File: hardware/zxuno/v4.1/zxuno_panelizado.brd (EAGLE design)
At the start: 190 x 150 mm, 2 parts

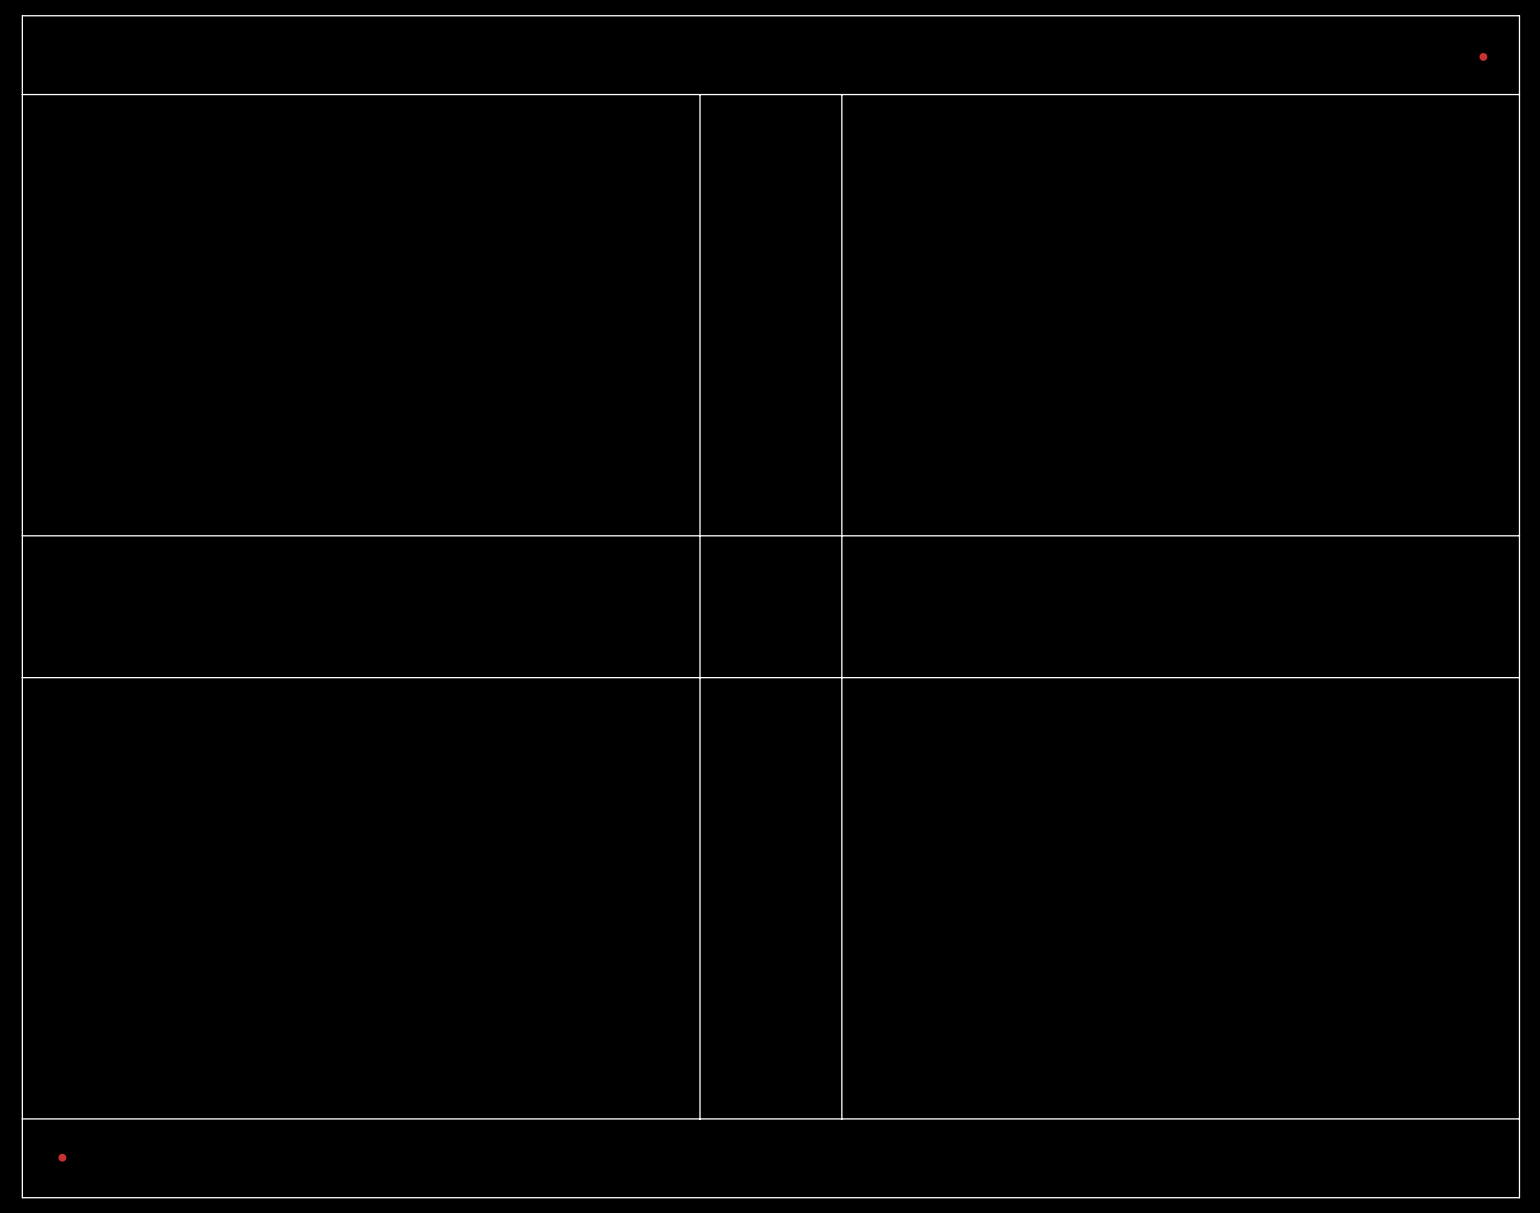
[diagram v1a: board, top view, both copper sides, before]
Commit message: Fin panelizado
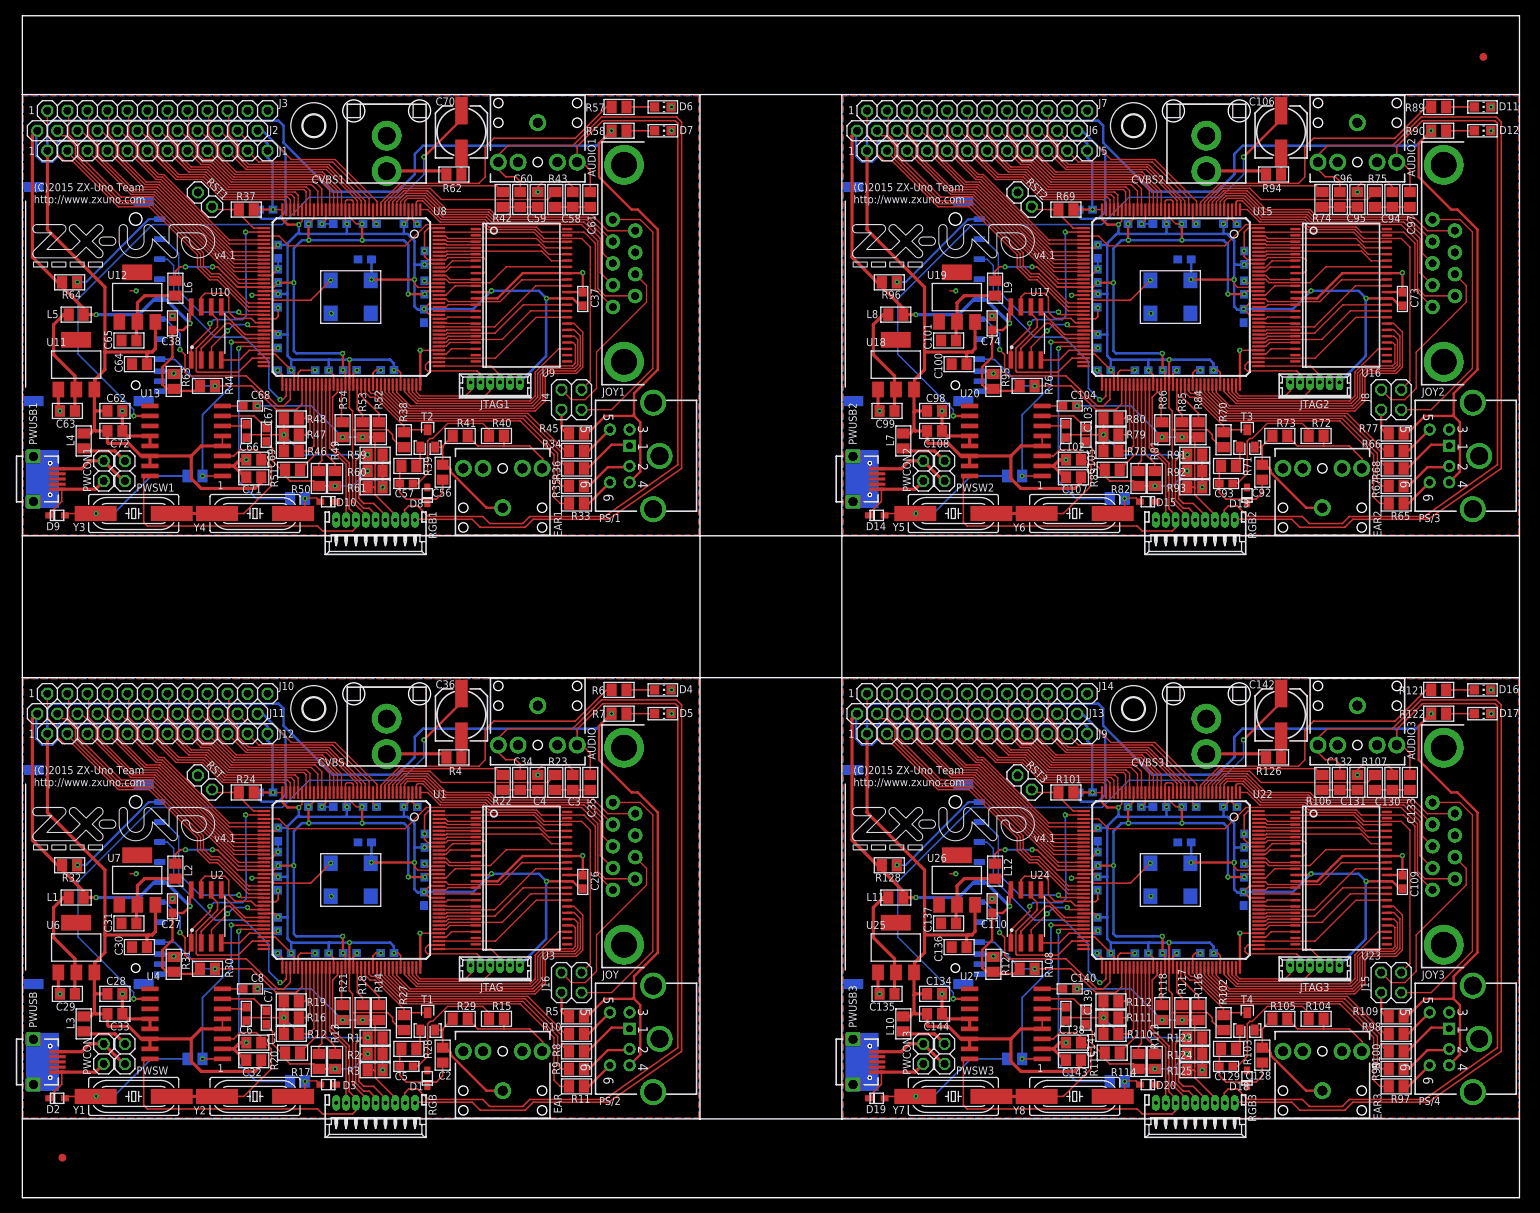
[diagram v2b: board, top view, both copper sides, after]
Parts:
- added AUDIO, AUDIO1, AUDIO2, AUDIO3: Audio, SparkFun-Connectors:AUDIO-JACK
- added C1, C105, C141, C69: 7.5pF, rcl:C0805
- added C10, C102, C103, C104, C109, C11, C110, C111, C112, C113, C114, C115, C116, C117, C118, C119, C12, C120, C121, C122, C123, C124, C125, C126, C127, C129, C13, C138, C139, C14, C140, C15, C16, C17, C18, C19, C20, C21, C22, C23, C24, C25, C26, C27, C37, C38, C39, C40, C41, C42, C43, C44, C45, C46, C47, C48, C49, C5, C50, C51, C52, C53, C54, C55, C57, C6, C66, C67, C68, C7, C73, C74, C75, C76, C77, C78, C79, C8, C80, C81, C82, C83, C84, C85, C86, C87, C88, C89, C9, C90, C91, C93: 100nF, rcl:C0603
- added C100, C101, C107, C108, C132, C133, C134, C135, C136, C137, C143, C144, C28, C29, C30, C31, C32, C33, C34, C35, C60, C61, C62, C63, C64, C65, C71, C72, C96, C97, C98, C99: 10uF, rcl:C0805
- added C106, C142, C36, C70: 220uF, rcl:153CLV-0605
- added C128, C130, C131, C2, C3, C4, C56, C58, C59, C92, C94, C95: 10nF, rcl:C0805
- added CVBS, CVBS1, CVBS2, CVBS3: RCA, uzebox:RCA
- added D1, D10, D13, D14, D15, D18, D19, D2, D20, D3, D8, D9: (no value), adafruit:SOD-323F
- added D11, D12, D16, D17, D4, D5, D6, D7: (no value), led:CHIP-LED0805
- added EAR, EAR1, EAR2, EAR3: EAR, SparkFun-Connectors:AUDIO-JACK
- added H1, H2, H3, H4: MOUNT-HOLE2.8, holes:2,8
- added J1, J10, J11, J12, J13, J14, J2, J3, J5, J6, J7, J9: (no value), pinhead:1X12
- added J15, J16, J4, J8: (no value), pinhead:2X02
- added JOY, JOY1, JOY2, JOY3: (no value), SparkFun-Connectors:DB9_MALE
- added JTAG, JTAG1, JTAG2, JTAG3: JTAG, con-molex:53047-06
- added L1, L10, L11, L12, L2, L3, L4, L5, L6, L7, L8, L9: (no value), rcl:M0805
- added PS/1, PS/2, PS/3, PS/4: PS/2 Keyb, ZX_UNO_0_14:DINC/MIN_TM/6_1PRIMARY
- added PWCON, PWCON1, PWCON2, PWCON3, PWSW, PWSW1, PWSW2, PWSW3, RST, RST1, RST2, RST3: (no value), pinhead:1X02
- added PWUSB, PWUSB1, PWUSB2, PWUSB3: MICROUSB, zxuno_rev_mcleod:MICRO_USB_1PRIMARY
- added R1, R123, R124, R125, R126, R2, R3, R4, R59, R60, R61, R62, R91, R92, R93, R94: 75, rcl:M0805
- added R10, R100, R104, R109, R11, R110, R113, R116, R12, R121, R122, R13, R14, R15, R33, R34, R35, R36, R40, R45, R46, R49, R5, R52, R57, R58, R6, R65, R66, R67, R68, R7, R72, R77, R78, R8, R81, R84, R89, R9, R90, R97, R98, R99: 510, rcl:M0805
- added R101, R106, R107, R112, R115, R118, R19, R20, R21, R22, R23, R24, R37, R42, R43, R48, R51, R54, R69, R74, R75, R80, R83, R86: 2K, rcl:M0805
- added R102, R103, R105, R108, R119, R120, R127, R128, R25, R26, R27, R28, R29, R30, R31, R32, R38, R39, R41, R44, R55, R56, R63, R64, R70, R71, R73, R76, R87, R88, R95, R96: 10K, rcl:M0805
- added R111, R114, R117, R16, R17, R18, R47, R50, R53, R79, R82, R85: 1K, rcl:M0805
- added RGB, RGB1, RGB2, RGB3: RGB, con-molex:53048-09
- added SDCARD, SDCARD1, SDCARD2, SDCARD3: (no value), zxuno_rev_mcleod:SDCMF-10915W010
- added T1, T2, T3, T4: BC846, transistor:SOT23
- added U1, U15, U22, U8: 6SLX9TQG144, xilinx_devices_V6:TQ144
- added U10, U17, U2, U24: FLASH-SPI-25XXSMD1, GadgetFactory:SO08-EIAJ
- added U11, U18, U25, U6: 3.3V, burr-brown:SOT223
- added U12, U19, U26, U7: 1.2V, burr-brown:SOT223
- added U13, U20, U27, U4: AD724, ad725:SO16W
- added U14, U21, U28, U5: 50MHz, ZX_UNO_0_15:SM/OSC_1PRIMARY
- added U16, U23, U3, U9: (no value), GadgetFactory:TSOP44-II
- added Y1, Y3, Y5, Y7: 3.58M, crystal:HC49UP
- added Y2, Y4, Y6, Y8: 4.43M, crystal:HC49UP
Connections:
- new net 1.2V: C10.2, C11.2, C12.2, C13.2, C9.2, L2.2, U1.P128, U1.P19, U1.P28, U1.P52, U1.P89
- new net 1.2V1: C39.2, C40.2, C41.2, C42.2, C43.2, L6.2, U8.P128, U8.P19, U8.P28, U8.P52, U8.P89
- new net 1.2V2: C75.2, C76.2, C77.2, C78.2, C79.2, L9.2, U15.P128, U15.P19, U15.P28, U15.P52, U15.P89
- new net 1.2V3: C111.2, C112.2, C113.2, C114.2, C115.2, L12.2, U22.P128, U22.P19, U22.P28, U22.P52, U22.P89
- new net 3.3V: C14.2, C15.2, C16.2, C17.2, C18.2, C19.2, C20.2, C21.2, C22.2, C23.2, C24.2, C25.2, C26.1, C27.2, J11.1, J12.12, JTAG.1, L1.2, R24.2, R27.2, R30.1, R31.2, R32.2, RGB.4, SDCARD.4, U1.P103, U1.P122, U1.P125, U1.P129, U1.P135, U1.P18, U1.P20, U1.P31, U1.P36, U1.P4, U1.P42, U1.P53, U1.P63, U1.P69, U1.P76, U1.P86, U1.P90, U2.8, U3.11, U3.33, U5.4
- new net 3.3V1: C37.1, C38.2, C44.2, C45.2, C46.2, C47.2, C48.2, C49.2, C50.2, C51.2, C52.2, C53.2, C54.2, C55.2, J1.12, J2.1, JTAG1.1, L5.2, R37.2, R38.2, R44.1, R63.2, R64.2, RGB1.4, SDCARD1.4, U10.8, U14.4, U8.P103, U8.P122, U8.P125, U8.P129, U8.P135, U8.P18, U8.P20, U8.P31, U8.P36, U8.P4, U8.P42, U8.P53, U8.P63, U8.P69, U8.P76, U8.P86, U8.P90, U9.11, U9.33
- new net 3.3V2: C73.1, C74.2, C80.2, C81.2, C82.2, C83.2, C84.2, C85.2, C86.2, C87.2, C88.2, C89.2, C90.2, C91.2, J5.12, J6.1, JTAG2.1, L8.2, R69.2, R70.2, R76.1, R95.2, R96.2, RGB2.4, SDCARD2.4, U15.P103, U15.P122, U15.P125, U15.P129, U15.P135, U15.P18, U15.P20, U15.P31, U15.P36, U15.P4, U15.P42, U15.P53, U15.P63, U15.P69, U15.P76, U15.P86, U15.P90, U16.11, U16.33, U17.8, U21.4
- new net 3.3V3: C109.1, C110.2, C116.2, C117.2, C118.2, C119.2, C120.2, C121.2, C122.2, C123.2, C124.2, C125.2, C126.2, C127.2, J13.1, J9.12, JTAG3.1, L11.2, R101.2, R102.2, R108.1, R127.2, R128.2, RGB3.4, SDCARD3.4, U22.P103, U22.P122, U22.P125, U22.P129, U22.P135, U22.P18, U22.P20, U22.P31, U22.P36, U22.P4, U22.P42, U22.P53, U22.P63, U22.P69, U22.P76, U22.P86, U22.P90, U23.11, U23.33, U24.8, U28.4
- new net 5V: C28.1, C30.1, C32.2, C33.2, J12.1, L3.2, PS/2.4, R5.1, R7.2, U4.14, U4.15, U4.4, U4.5, U6.3, U7.3
- new net 5V1: C62.1, C64.1, C71.2, C72.2, J1.1, L4.2, PS/1.4, R45.1, R58.2, U11.3, U12.3, U13.14, U13.15, U13.4, U13.5
- new net 5V2: C100.1, C107.2, C108.2, C98.1, J5.1, L7.2, PS/3.4, R77.1, R90.2, U18.3, U19.3, U20.14, U20.15, U20.4, U20.5
- new net 5V3: C134.1, C136.1, C143.2, C144.2, J9.1, L10.2, PS/4.4, R109.1, R122.2, U25.3, U26.3, U27.14, U27.15, U27.4, U27.5
- new net AUDIO_LEFT: R22.2, U1.P10
- new net AUDIO_LEFT1: R42.2, U8.P10
- new net AUDIO_LEFT2: R74.2, U15.P10
- new net AUDIO_LEFT3: R106.2, U22.P10
- new net AUDIO_RIGHT: R23.2, U1.P9
- new net AUDIO_RIGHT1: R43.2, U8.P9
- new net AUDIO_RIGHT2: R75.2, U15.P9
- new net AUDIO_RIGHT3: R107.2, U22.P9
- new net B: C8.2, R14.1, R18.1, R21.1, R3.1, RGB.7
- new net B0: R21.2, U1.P88
- new net B1: R18.2, U1.P92
- new net B10: C104.2, R84.1, R85.1, R86.1, R93.1, RGB2.7
- new net B11: R118.2, U22.P88
- new net B12: R117.2, U22.P92
- new net B13: R116.2, U22.P93
- new net B14: C140.2, R116.1, R117.1, R118.1, R125.1, RGB3.7
- new net B2: R14.2, U1.P93
- new net B3: R54.2, U8.P88
- new net B4: R53.2, U8.P92
- new net B5: R52.2, U8.P93
- new net B6: C68.2, R52.1, R53.1, R54.1, R61.1, RGB1.7
- new net B7: R86.2, U15.P88
- new net B8: R85.2, U15.P92
- new net B9: R84.2, U15.P93
- new net CLK: U1.P55, U5.3
- new net CLK1: U14.3, U8.P55
- new net CLK2: U15.P55, U21.3
- new net CLK3: U22.P55, U28.3
- new net CSYNC: RGB.3, U1.P87, U4.16
- new net CSYNC1: RGB1.3, U13.16, U8.P87
- new net CSYNC2: RGB2.3, U15.P87, U20.16
- new net CSYNC3: RGB3.3, U22.P87, U27.16
- new net EAR: R27.1, T1.3, U1.P94
- new net EAR1: R38.1, T2.3, U8.P94
- new net EAR2: R70.1, T3.3, U15.P94
- new net EAR3: R102.1, T4.3, U22.P94
- new net EXT1: J1.2, U8.P57
- new net EXT10: J12.3, U1.P50
- new net EXT100: J9.5, U22.P43
- new net EXT101: J13.5, U22.P41
- new net EXT102: J14.5, U22.P40
- new net EXT103: J9.6, U22.P35
- new net EXT104: J13.6, U22.P34
- new net EXT105: J14.6, U22.P33
- new net EXT106: J9.7, U22.P32
- new net EXT107: J13.7, U22.P30
- new net EXT108: J14.7, U22.P29
- new net EXT109: J9.8, U22.P27
- new net EXT11: J11.3, U1.P48
- new net EXT110: J13.8, U22.P26
- new net EXT111: J14.8, U22.P24
- new net EXT112: J9.9, U22.P23
- new net EXT113: J13.9, U22.P22
- new net EXT114: J14.9, U22.P21
- new net EXT115: J9.10, U22.P17
- new net EXT116: J13.10, U22.P16
- new net EXT117: J14.10, U22.P15
- new net EXT118: J9.11, U22.P14
- new net EXT119: J13.11, U22.P12
- new net EXT12: J10.3, U1.P47
- new net EXT120: J14.1, U22.P58
- new net EXT13: J12.4, U1.P46
- new net EXT14: J11.4, U1.P45
- new net EXT15: J10.4, U1.P44
- new net EXT16: J12.5, U1.P43
- new net EXT17: J11.5, U1.P41
- new net EXT18: J10.5, U1.P40
- new net EXT19: J12.6, U1.P35
- new net EXT2: J2.2, U8.P56
- new net EXT20: J11.6, U1.P34
- new net EXT21: J10.6, U1.P33
- new net EXT22: J12.7, U1.P32
- new net EXT23: J11.7, U1.P30
- new net EXT24: J10.7, U1.P29
- new net EXT25: J12.8, U1.P27
- new net EXT26: J11.8, U1.P26
- new net EXT27: J10.8, U1.P24
- new net EXT28: J12.9, U1.P23
- new net EXT29: J11.9, U1.P22
- new net EXT3: J3.2, U8.P51
- new net EXT30: J10.9, U1.P21
- new net EXT31: J12.10, U1.P17
- new net EXT32: J11.10, U1.P16
- new net EXT33: J10.10, U1.P15
- new net EXT34: J12.11, U1.P14
- new net EXT35: J11.11, U1.P12
- new net EXT36: J3.3, U8.P47
- new net EXT37: J1.4, U8.P46
- new net EXT38: J2.4, U8.P45
- new net EXT39: J3.4, U8.P44
- new net EXT4: J1.3, U8.P50
- new net EXT40: J1.5, U8.P43
- new net EXT41: J2.5, U8.P41
- new net EXT42: J3.5, U8.P40
- new net EXT43: J1.6, U8.P35
- new net EXT44: J2.6, U8.P34
- new net EXT45: J3.6, U8.P33
- new net EXT46: J1.7, U8.P32
- new net EXT47: J2.7, U8.P30
- new net EXT48: J3.7, U8.P29
- new net EXT49: J1.8, U8.P27
- new net EXT5: J2.3, U8.P48
- new net EXT50: J2.8, U8.P26
- new net EXT51: J3.8, U8.P24
- new net EXT52: J1.9, U8.P23
- new net EXT53: J2.9, U8.P22
- new net EXT54: J3.9, U8.P21
- new net EXT55: J1.10, U8.P17
- new net EXT56: J2.10, U8.P16
- new net EXT57: J3.10, U8.P15
- new net EXT58: J1.11, U8.P14
- new net EXT59: J2.11, U8.P12
- new net EXT6: J10.1, U1.P58
- new net EXT60: J3.1, U8.P58
- new net EXT61: J5.2, U15.P57
- new net EXT62: J6.2, U15.P56
- new net EXT63: J7.2, U15.P51
- new net EXT64: J5.3, U15.P50
- new net EXT65: J6.3, U15.P48
- new net EXT66: J7.3, U15.P47
- new net EXT67: J5.4, U15.P46
- new net EXT68: J6.4, U15.P45
- new net EXT69: J7.4, U15.P44
- new net EXT7: J12.2, U1.P57
- new net EXT70: J5.5, U15.P43
- new net EXT71: J6.5, U15.P41
- new net EXT72: J7.5, U15.P40
- new net EXT73: J5.6, U15.P35
- new net EXT74: J6.6, U15.P34
- new net EXT75: J7.6, U15.P33
- new net EXT76: J5.7, U15.P32
- new net EXT77: J6.7, U15.P30
- new net EXT78: J7.7, U15.P29
- new net EXT79: J5.8, U15.P27
- new net EXT8: J11.2, U1.P56
- new net EXT80: J6.8, U15.P26
- new net EXT81: J7.8, U15.P24
- new net EXT82: J5.9, U15.P23
- new net EXT83: J6.9, U15.P22
- new net EXT84: J7.9, U15.P21
- new net EXT85: J5.10, U15.P17
- new net EXT86: J6.10, U15.P16
- new net EXT87: J7.10, U15.P15
- new net EXT88: J5.11, U15.P14
- new net EXT89: J6.11, U15.P12
- new net EXT9: J10.2, U1.P51
- new net EXT90: J7.1, U15.P58
- new net EXT91: J9.2, U22.P57
- new net EXT92: J13.2, U22.P56
- new net EXT93: J14.2, U22.P51
- new net EXT94: J9.3, U22.P50
- new net EXT95: J13.3, U22.P48
- new net EXT96: J14.3, U22.P47
- new net EXT97: J9.4, U22.P46
- new net EXT98: J13.4, U22.P45
- new net EXT99: J14.4, U22.P44
- new net FLASH_CS: U1.P38, U2.1
- new net FLASH_CS1: U10.1, U8.P38
- new net FLASH_CS2: U15.P38, U17.1
- new net FLASH_CS3: U22.P38, U24.1
- new net FLASH_HOLD: U1.P61, U2.7
- new net FLASH_HOLD1: U10.7, U8.P61
- new net FLASH_HOLD2: U15.P61, U17.7
- new net FLASH_HOLD3: U22.P61, U24.7
- new net FLASH_MISO: U1.P65, U2.2
- new net FLASH_MISO1: U10.2, U8.P65
- new net FLASH_MISO2: U15.P65, U17.2
- new net FLASH_MISO3: U22.P65, U24.2
- new net FLASH_MOSI: U1.P64, U2.5
- new net FLASH_MOSI1: U10.5, U8.P64
- new net FLASH_MOSI2: U15.P64, U17.5
- new net FLASH_MOSI3: U22.P64, U24.5
- new net FLASH_SCK: U1.P70, U2.6
- new net FLASH_SCK1: U10.6, U8.P70
- new net FLASH_SCK2: U15.P70, U17.6
- new net FLASH_SCK3: U22.P70, U24.6
- new net FLASH_WP: U1.P62, U2.3
- new net FLASH_WP1: U10.3, U8.P62
- new net FLASH_WP2: U15.P62, U17.3
- new net FLASH_WP3: U22.P62, U24.3
- new net G: C7.2, R13.1, R17.1, R2.1, R20.1, RGB.6
- new net G0: R20.2, U1.P82
- new net G1: R17.2, U1.P83
- new net G10: C103.2, R81.1, R82.1, R83.1, R92.1, RGB2.6
- new net G11: R115.2, U22.P82
- new net G12: R114.2, U22.P83
- new net G13: R113.2, U22.P84
- new net G14: C139.2, R113.1, R114.1, R115.1, R124.1, RGB3.6
- new net G2: R13.2, U1.P84
- new net G3: R51.2, U8.P82
- new net G4: R50.2, U8.P83
- new net G5: R49.2, U8.P84
- new net G6: C67.2, R49.1, R50.1, R51.1, R60.1, RGB1.6
- new net G7: R83.2, U15.P82
- new net G8: R82.2, U15.P83
- new net G9: R81.2, U15.P84
- new net GND: AUDIO.SLEEVE, C1.2, C10.1, C11.1, C12.1, C13.1, C14.1, C15.1, C16.1, C17.1, C18.1, C19.1, C2.2, C20.1, C21.1, C22.1, C23.1, C24.1, C25.1, C26.2, C27.1, C28.2, C29.2, C3.2, C30.2, C31.2, C32.1, C33.1, C4.2, C9.1, CVBS.GND, D1.A, D2.C, D3.C, D4.C, D5.C, EAR.SLEEVE, J10.12, J11.12, JOY.8, JTAG.2, PS/2.3, PWCON.1, PWUSB.5, R1.2, R2.2, R29.2, R3.2, RGB.1, RST.1, SDCARD.3, SDCARD.6, SDCARD.M1, SDCARD.M2, SDCARD.M3, SDCARD.M4, T1.2, U1.P108, U1.P113, U1.P13, U1.P130, U1.P136, U1.P144, U1.P25, U1.P3, U1.P49, U1.P54, U1.P60, U1.P68, U1.P73, U1.P77, U1.P91, U1.P96, U2.4, U3.12, U3.34, U3.37, U3.8, U4.12, U4.13, U4.2, U5.2, U6.1, U7.1
- new net GND1: AUDIO1.SLEEVE, C37.2, C38.1, C39.1, C40.1, C41.1, C42.1, C43.1, C44.1, C45.1, C46.1, C47.1, C48.1, C49.1, C50.1, C51.1, C52.1, C53.1, C54.1, C55.1, C56.2, C58.2, C59.2, C62.2, C63.2, C64.2, C65.2, C69.2, C71.1, C72.1, CVBS1.GND, D10.C, D6.C, D7.C, D8.A, D9.C, EAR1.SLEEVE, J2.12, J3.12, JOY1.8, JTAG1.2, PS/1.3, PWCON1.1, PWUSB1.5, R41.2, R59.2, R60.2, R61.2, RGB1.1, RST1.1, SDCARD1.3, SDCARD1.6, SDCARD1.M1, SDCARD1.M2, SDCARD1.M3, SDCARD1.M4, T2.2, U10.4, U11.1, U12.1, U13.12, U13.13, U13.2, U14.2, U8.P108, U8.P113, U8.P13, U8.P130, U8.P136, U8.P144, U8.P25, U8.P3, U8.P49, U8.P54, U8.P60, U8.P68, U8.P73, U8.P77, U8.P91, U8.P96, U9.12, U9.34, U9.37, U9.8
- new net GND2: AUDIO2.SLEEVE, C100.2, C101.2, C105.2, C107.1, C108.1, C73.2, C74.1, C75.1, C76.1, C77.1, C78.1, C79.1, C80.1, C81.1, C82.1, C83.1, C84.1, C85.1, C86.1, C87.1, C88.1, C89.1, C90.1, C91.1, C92.2, C94.2, C95.2, C98.2, C99.2, CVBS2.GND, D11.C, D12.C, D13.A, D14.C, D15.C, EAR2.SLEEVE, J6.12, J7.12, JOY2.8, JTAG2.2, PS/3.3, PWCON2.1, PWUSB2.5, R73.2, R91.2, R92.2, R93.2, RGB2.1, RST2.1, SDCARD2.3, SDCARD2.6, SDCARD2.M1, SDCARD2.M2, SDCARD2.M3, SDCARD2.M4, T3.2, U15.P108, U15.P113, U15.P13, U15.P130, U15.P136, U15.P144, U15.P25, U15.P3, U15.P49, U15.P54, U15.P60, U15.P68, U15.P73, U15.P77, U15.P91, U15.P96, U16.12, U16.34, U16.37, U16.8, U17.4, U18.1, U19.1, U20.12, U20.13, U20.2, U21.2
- new net GND3: AUDIO3.SLEEVE, C109.2, C110.1, C111.1, C112.1, C113.1, C114.1, C115.1, C116.1, C117.1, C118.1, C119.1, C120.1, C121.1, C122.1, C123.1, C124.1, C125.1, C126.1, C127.1, C128.2, C130.2, C131.2, C134.2, C135.2, C136.2, C137.2, C141.2, C143.1, C144.1, CVBS3.GND, D16.C, D17.C, D18.A, D19.C, D20.C, EAR3.SLEEVE, J13.12, J14.12, JOY3.8, JTAG3.2, PS/4.3, PWCON3.1, PWUSB3.5, R105.2, R123.2, R124.2, R125.2, RGB3.1, RST3.1, SDCARD3.3, SDCARD3.6, SDCARD3.M1, SDCARD3.M2, SDCARD3.M3, SDCARD3.M4, T4.2, U22.P108, U22.P113, U22.P13, U22.P130, U22.P136, U22.P144, U22.P25, U22.P3, U22.P49, U22.P54, U22.P60, U22.P68, U22.P73, U22.P77, U22.P91, U22.P96, U23.12, U23.34, U23.37, U23.8, U24.4, U25.1, U26.1, U27.12, U27.13, U27.2, U28.2
- new net JOY_DOWN: JOY.2, U1.P5
- new net JOY_DOWN1: JOY1.2, U8.P5
- new net JOY_DOWN2: JOY2.2, U15.P5
- new net JOY_DOWN3: JOY3.2, U22.P5
- new net JOY_FIRE1: JOY.6, U1.P2
- new net JOY_FIRE10: JOY3.6, U22.P2
- new net JOY_FIRE11: JOY3.9, U22.P8
- new net JOY_FIRE12: J15.1, U22.P39
- new net JOY_FIRE2: JOY.9, U1.P8
- new net JOY_FIRE3: J16.1, U1.P39
- new net JOY_FIRE4: JOY1.6, U8.P2
- new net JOY_FIRE5: JOY1.9, U8.P8
- new net JOY_FIRE6: J4.1, U8.P39
- new net JOY_FIRE7: JOY2.6, U15.P2
- new net JOY_FIRE8: JOY2.9, U15.P8
- new net JOY_FIRE9: J8.1, U15.P39
- new net JOY_LEFT: JOY.3, U1.P6
- new net JOY_LEFT1: JOY1.3, U8.P6
- new net JOY_LEFT2: JOY2.3, U15.P6
- new net JOY_LEFT3: JOY3.3, U22.P6
- new net JOY_RIGHT: JOY.4, U1.P7
- new net JOY_RIGHT1: JOY1.4, U8.P7
- new net JOY_RIGHT2: JOY2.4, U15.P7
- new net JOY_RIGHT3: JOY3.4, U22.P7
- new net JOY_UP: JOY.1, U1.P1
- new net JOY_UP1: JOY1.1, U8.P1
- new net JOY_UP2: JOY2.1, U15.P1
- new net JOY_UP3: JOY3.1, U22.P1
- new net L-OUT: AUDIO.TIP, C34.2, RGB.9
- new net L-OUT1: AUDIO1.TIP, C60.2, RGB1.9
- new net L-OUT2: AUDIO2.TIP, C96.2, RGB2.9
- new net L-OUT3: AUDIO3.TIP, C132.2, RGB3.9
- new net LED: R6.2, U1.P11
- new net LED1: R57.2, U8.P11
- new net LED2: R89.2, U15.P11
- new net LED3: R121.2, U22.P11
- new net N$1: PS/2.6, R11.1
- new net N$10: C3.1, C35.1, R23.1
- new net N$100: C135.1, L11.1, U25.2
- new net N$101: C137.1, L12.1, U26.2
- new net N$102: C139.1, U27.7
- new net N$103: C138.1, U27.6
- new net N$104: C141.1, U27.3, Y7.2, Y8.2
- new net N$105: D20.A, R120.1, Y8.1
- new net N$106: D19.A, R119.2, Y7.1
- new net N$107: C142.+, U27.10
- new net N$108: C140.1, U27.8
- new net N$109: C142.-, R126.1
- new net N$11: C34.1, C4.1, R22.1
- new net N$110: CVBS3.SIG, R126.2
- new net N$111: D16.A, R121.1
- new net N$112: D17.A, R122.1
- new net N$113: R101.1, RST3.2, U22.P37
- new net N$114: R127.1, SDCARD3.8
- new net N$115: R128.1, SDCARD3.9
- new net N$116: J15.4, R109.2
- new net N$12: PWCON.2, PWSW.2, PWUSB.1
- new net N$13: L3.1, PWSW.1
- new net N$14: C29.1, L1.1, U6.2
- new net N$15: J16.4, R5.2
- new net N$16: PS/1.6, R33.1
- new net N$17: C31.1, L2.1, U7.2
- new net N$18: R31.1, SDCARD.8
- new net N$19: C8.1, U4.8
- new net N$2: PS/2.5, R10.1
- new net N$20: R32.1, SDCARD.9
- new net N$21: C7.1, U4.7
- new net N$22: C6.1, U4.6
- new net N$23: C1.1, U4.3, Y1.2, Y2.2
- new net N$24: D3.A, R26.1, Y2.1
- new net N$25: D2.A, R25.2, Y1.1
- new net N$26: C36.+, U4.10
- new net N$27: C36.-, R4.1
- new net N$28: CVBS.SIG, R4.2
- new net N$29: PS/1.5, R34.1
- new net N$3: PS/2.2, R9.1
- new net N$30: PS/1.2, R35.1
- new net N$31: D4.A, R6.1
- new net N$32: D5.A, R7.1
- new net N$33: PS/1.1, R36.1
- new net N$34: R39.2, T2.1
- new net N$35: C56.1, C57.1, D8.C, R39.1
- new net N$36: C57.2, R40.2
- new net N$37: EAR1.TIP, R40.1, R41.1
- new net N$38: C58.1, C61.1, R43.1
- new net N$39: C59.1, C60.1, R42.1
- new net N$4: PS/2.1, R8.1
- new net N$40: PWCON1.2, PWSW1.2, PWUSB1.1
- new net N$41: L4.1, PWSW1.1
- new net N$42: C63.1, L5.1, U11.2
- new net N$43: C65.1, L6.1, U12.2
- new net N$44: C67.1, U13.7
- new net N$45: C66.1, U13.6
- new net N$46: C69.1, U13.3, Y3.2, Y4.2
- new net N$47: D10.A, R56.1, Y4.1
- new net N$48: D9.A, R55.2, Y3.1
- new net N$49: C70.+, U13.10
- new net N$5: R24.1, RST.2, U1.P37
- new net N$50: C68.1, U13.8
- new net N$51: C70.-, R62.1
- new net N$52: CVBS1.SIG, R62.2
- new net N$53: D6.A, R57.1
- new net N$54: D7.A, R58.1
- new net N$55: R37.1, RST1.2, U8.P37
- new net N$56: R63.1, SDCARD1.8
- new net N$57: R64.1, SDCARD1.9
- new net N$58: J4.4, R45.2
- new net N$59: PS/3.6, R65.1
- new net N$6: R28.2, T1.1
- new net N$60: PS/3.5, R66.1
- new net N$61: PS/3.2, R67.1
- new net N$62: PS/3.1, R68.1
- new net N$63: R71.2, T3.1
- new net N$64: C92.1, C93.1, D13.C, R71.1
- new net N$65: C93.2, R72.2
- new net N$66: EAR2.TIP, R72.1, R73.1
- new net N$67: C94.1, C97.1, R75.1
- new net N$68: C95.1, C96.1, R74.1
- new net N$69: PWCON2.2, PWSW2.2, PWUSB2.1
- new net N$7: C2.1, C5.1, D1.C, R28.1
- new net N$70: L7.1, PWSW2.1
- new net N$71: C99.1, L8.1, U18.2
- new net N$72: C101.1, L9.1, U19.2
- new net N$73: C103.1, U20.7
- new net N$74: C102.1, U20.6
- new net N$75: C105.1, U20.3, Y5.2, Y6.2
- new net N$76: D15.A, R88.1, Y6.1
- new net N$77: D14.A, R87.2, Y5.1
- new net N$78: C106.+, U20.10
- new net N$79: C104.1, U20.8
- new net N$8: C5.2, R15.2
- new net N$80: C106.-, R94.1
- new net N$81: CVBS2.SIG, R94.2
- new net N$82: D11.A, R89.1
- new net N$83: D12.A, R90.1
- new net N$84: R69.1, RST2.2, U15.P37
- new net N$85: R95.1, SDCARD2.8
- new net N$86: R96.1, SDCARD2.9
- new net N$87: J8.4, R77.2
- new net N$88: PS/4.6, R97.1
- new net N$89: PS/4.5, R98.1
- new net N$9: EAR.TIP, R15.1, R29.1
- new net N$90: PS/4.2, R99.1
- new net N$91: PS/4.1, R100.1
- new net N$92: R103.2, T4.1
- new net N$93: C128.1, C129.1, D18.C, R103.1
- new net N$94: C129.2, R104.2
- new net N$95: EAR3.TIP, R104.1, R105.1
- new net N$96: C130.1, C133.1, R107.1
- new net N$97: C131.1, C132.1, R106.1
- new net N$98: PWCON3.2, PWSW3.2, PWUSB3.1
- new net N$99: L10.1, PWSW3.1
- new net PIN1: J4.3, JOY1.7
- new net PIN2: J4.2, JOY1.5
- new net PIN3: J8.3, JOY2.7
- new net PIN4: J8.2, JOY2.5
- new net PIN5: J16.2, JOY.5
- new net PIN6: J15.3, JOY3.7
- new net PIN7: J16.3, JOY.7
- new net PIN8: J15.2, JOY3.5
- new net PS2_CLK: R10.2, U1.P99
- new net PS2_CLK1: R34.2, U8.P99
- new net PS2_CLK2: R66.2, U15.P99
- new net PS2_CLK3: R98.2, U22.P99
- new net PS2_DATA: R8.2, U1.P98
- new net PS2_DATA1: R36.2, U8.P98
- new net PS2_DATA2: R68.2, U15.P98
- new net PS2_DATA3: R100.2, U22.P98
- new net PS2_PIN1: R33.2, U8.P95
- new net PS2_PIN2: R9.2, U1.P97
- new net PS2_PIN3: R35.2, U8.P97
- new net PS2_PIN4: R65.2, U15.P95
- new net PS2_PIN5: R67.2, U15.P97
- new net PS2_PIN6: R11.2, U1.P95
- new net PS2_PIN7: R97.2, U22.P95
- new net PS2_PIN8: R99.2, U22.P97
- new net R: C6.2, R1.1, R12.1, R16.1, R19.1, RGB.5
- new net R-OUT: AUDIO.RING, C35.2, RGB.8
- new net R-OUT1: AUDIO1.RING, C61.2, RGB1.8
- new net R-OUT2: AUDIO2.RING, C97.2, RGB2.8
- new net R-OUT3: AUDIO3.RING, C133.2, RGB3.8
- new net R0: R19.2, U1.P79
- new net R1: R16.2, U1.P80
- new net R10: C102.2, R78.1, R79.1, R80.1, R91.1, RGB2.5
- new net R11: R112.2, U22.P79
- new net R12: R111.2, U22.P80
- new net R13: R110.2, U22.P81
- new net R14: C138.2, R110.1, R111.1, R112.1, R123.1, RGB3.5
- new net R2: R12.2, U1.P81
- new net R3: R48.2, U8.P79
- new net R4: R47.2, U8.P80
- new net R5: R46.2, U8.P81
- new net R6: C66.2, R46.1, R47.1, R48.1, R59.1, RGB1.5
- new net R7: R80.2, U15.P79
- new net R8: R79.2, U15.P80
- new net R9: R78.2, U15.P81
- new net SD_CS: SDCARD.1, U1.P59
- new net SD_CS1: SDCARD1.1, U8.P59
- new net SD_CS2: SDCARD2.1, U15.P59
- new net SD_CS3: SDCARD3.1, U22.P59
- new net SD_MISO: R30.2, SDCARD.7, U1.P78
- new net SD_MISO1: R44.2, SDCARD1.7, U8.P78
- new net SD_MISO2: R76.2, SDCARD2.7, U15.P78
- new net SD_MISO3: R108.2, SDCARD3.7, U22.P78
- new net SD_MOSI: SDCARD.2, U1.P74
- new net SD_MOSI1: SDCARD1.2, U8.P74
- new net SD_MOSI2: SDCARD2.2, U15.P74
- new net SD_MOSI3: SDCARD3.2, U22.P74
- new net SD_SCK: SDCARD.5, U1.P75
- new net SD_SCK1: SDCARD1.5, U8.P75
- new net SD_SCK2: SDCARD2.5, U15.P75
- new net SD_SCK3: SDCARD3.5, U22.P75
- new net STDN: R25.1, U1.P66, U4.1
- new net STDN1: R55.1, U13.1, U8.P66
- new net STDN2: R87.1, U15.P66, U20.1
- new net STDN3: R119.1, U22.P66, U27.1
- new net STDNB: R26.2, U1.P67
- new net STDNB1: R56.2, U8.P67
- new net STDNB2: R88.2, U15.P67
- new net STDNB3: R120.2, U22.P67
- new net TCK: JTAG.3, U1.P109
- new net TCK1: JTAG1.3, U8.P109
- new net TCK2: JTAG2.3, U15.P109
- new net TCK3: JTAG3.3, U22.P109
- new net TDI: JTAG.5, U1.P110
- new net TDI1: JTAG1.5, U8.P110
- new net TDI2: JTAG2.5, U15.P110
- new net TDI3: JTAG3.5, U22.P110
- new net TDO: JTAG.4, U1.P106
- new net TDO1: JTAG1.4, U8.P106
- new net TDO2: JTAG2.4, U15.P106
- new net TDO3: JTAG3.4, U22.P106
- new net TMS: JTAG.6, U1.P107
- new net TMS1: JTAG1.6, U8.P107
- new net TMS2: JTAG2.6, U15.P107
- new net TMS3: JTAG3.6, U22.P107
- new net VSYNC: RGB.2, U1.P85
- new net VSYNC1: RGB1.2, U8.P85
- new net VSYNC2: RGB2.2, U15.P85
- new net VSYNC3: RGB3.2, U22.P85
- new net WR: U1.P121, U3.15
- new net WR1: U8.P121, U9.15
- new net WR2: U15.P121, U16.15
- new net WR3: U22.P121, U23.15
- new net XA0: U1.P141, U3.3
- new net XA1: U1.P139, U3.4
- new net XA10: U1.P104, U3.26
- new net XA11: U1.P102, U3.27
- new net XA12: U1.P101, U3.28
- new net XA13: U1.P100, U3.29
- new net XA14: U1.P111, U3.30
- new net XA15: U1.P131, U3.38
- new net XA16: U1.P138, U3.39
- new net XA17: U1.P140, U3.40
- new net XA18: U1.P142, U3.41
- new net XA19: U1.P105, U3.25
- new net XA2: U1.P137, U3.5
- new net XA20: U1.P143, U3.42
- new net XA21: U8.P141, U9.3
- new net XA22: U8.P137, U9.5
- new net XA23: U8.P134, U9.6
- new net XA24: U8.P133, U9.7
- new net XA25: U8.P120, U9.16
- new net XA26: U8.P118, U9.17
- new net XA27: U8.P116, U9.18
- new net XA28: U8.P114, U9.19
- new net XA29: U8.P112, U9.20
- new net XA3: U1.P134, U3.6
- new net XA30: U8.P104, U9.26
- new net XA31: U8.P102, U9.27
- new net XA32: U8.P101, U9.28
- new net XA33: U8.P100, U9.29
- new net XA34: U8.P111, U9.30
- new net XA35: U8.P131, U9.38
- new net XA36: U8.P138, U9.39
- new net XA37: U8.P140, U9.40
- new net XA38: U8.P142, U9.41
- new net XA39: U8.P105, U9.25
- new net XA4: U1.P133, U3.7
- new net XA40: U8.P143, U9.42
- new net XA41: U8.P139, U9.4
- new net XA42: U15.P141, U16.3
- new net XA43: U15.P137, U16.5
- new net XA44: U15.P134, U16.6
- new net XA45: U15.P133, U16.7
- new net XA46: U15.P120, U16.16
- new net XA47: U15.P118, U16.17
- new net XA48: U15.P116, U16.18
- new net XA49: U15.P114, U16.19
- new net XA5: U1.P120, U3.16
- new net XA50: U15.P112, U16.20
- new net XA51: U15.P104, U16.26
- new net XA52: U15.P102, U16.27
- new net XA53: U15.P101, U16.28
- new net XA54: U15.P100, U16.29
- new net XA55: U15.P111, U16.30
- new net XA56: U15.P131, U16.38
- new net XA57: U15.P138, U16.39
- new net XA58: U15.P140, U16.40
- new net XA59: U15.P142, U16.41
- new net XA6: U1.P118, U3.17
- new net XA60: U15.P105, U16.25
- new net XA61: U15.P143, U16.42
- new net XA62: U15.P139, U16.4
- new net XA63: U22.P141, U23.3
- new net XA64: U22.P137, U23.5
- new net XA65: U22.P134, U23.6
- new net XA66: U22.P133, U23.7
- new net XA67: U22.P120, U23.16
- new net XA68: U22.P118, U23.17
- new net XA69: U22.P116, U23.18
- new net XA7: U1.P116, U3.18
- new net XA70: U22.P114, U23.19
- new net XA71: U22.P112, U23.20
- new net XA72: U22.P104, U23.26
- new net XA73: U22.P102, U23.27
- new net XA74: U22.P101, U23.28
- new net XA75: U22.P100, U23.29
- new net XA76: U22.P111, U23.30
- new net XA77: U22.P131, U23.38
- new net XA78: U22.P138, U23.39
- new net XA79: U22.P140, U23.40
- new net XA8: U1.P114, U3.19
- new net XA80: U22.P142, U23.41
- new net XA81: U22.P105, U23.25
- new net XA82: U22.P143, U23.42
- new net XA83: U22.P139, U23.4
- new net XA9: U1.P112, U3.20
- new net XD0: U1.P132, U3.9
- new net XD1: U1.P127, U3.10
- new net XD10: U8.P124, U9.13
- new net XD11: U8.P123, U9.14
- new net XD12: U8.P115, U9.31
- new net XD13: U8.P117, U9.32
- new net XD14: U8.P119, U9.35
- new net XD15: U8.P126, U9.36
- new net XD16: U15.P132, U16.9
- new net XD17: U15.P127, U16.10
- new net XD18: U15.P124, U16.13
- new net XD19: U15.P123, U16.14
- new net XD2: U1.P124, U3.13
- new net XD20: U15.P115, U16.31
- new net XD21: U15.P117, U16.32
- new net XD22: U15.P119, U16.35
- new net XD23: U15.P126, U16.36
- new net XD24: U22.P132, U23.9
- new net XD25: U22.P127, U23.10
- new net XD26: U22.P124, U23.13
- new net XD27: U22.P123, U23.14
- new net XD28: U22.P115, U23.31
- new net XD29: U22.P117, U23.32
- new net XD3: U1.P123, U3.14
- new net XD30: U22.P119, U23.35
- new net XD31: U22.P126, U23.36
- new net XD4: U1.P115, U3.31
- new net XD5: U1.P117, U3.32
- new net XD6: U1.P119, U3.35
- new net XD7: U1.P126, U3.36
- new net XD8: U8.P132, U9.9
- new net XD9: U8.P127, U9.10
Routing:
- net 3.3V1: track 0.00 -> 287.8 mm, vias 0 -> 19
- net 3.3V: track 0.00 -> 287.8 mm, vias 0 -> 19
- net 3.3V3: track 0.00 -> 287.8 mm, vias 0 -> 19
- net 3.3V2: track 0.00 -> 287.8 mm, vias 0 -> 19
- net 5V3: track 0.00 -> 233.3 mm, vias 0 -> 1
- net 5V1: track 0.00 -> 233.3 mm, vias 0 -> 1
- net 5V: track 0.00 -> 233.3 mm, vias 0 -> 1
- net 5V2: track 0.00 -> 233.3 mm, vias 0 -> 1
- net GND2: track 0.00 -> 149.1 mm, vias 0 -> 25
- net GND3: track 0.00 -> 149.1 mm, vias 0 -> 25
- net GND1: track 0.00 -> 149.1 mm, vias 0 -> 25
- net GND: track 0.00 -> 149.1 mm, vias 0 -> 25
- net L-OUT3: track 0.00 -> 112.9 mm
- net L-OUT2: track 0.00 -> 112.9 mm
- net L-OUT1: track 0.00 -> 112.9 mm
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- added copper zone on layer 1, net GND
- added copper zone on layer 16, net GND
- added copper zone on layer 1, net GND1
- added copper zone on layer 16, net GND1
- added copper zone on layer 1, net GND2
- added copper zone on layer 16, net GND2
- added copper zone on layer 1, net GND3
- added copper zone on layer 16, net GND3
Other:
- board text added: "(C)2015 ZX-Uno Team http://www.zxuno.com"
- board text added: "1"
- board text added: "AUDIO"
- board text added: "C1"
- board text added: "C10"
- board text added: "C11"
- board text added: "C12"
- board text added: "C13"
- board text added: "C14"
- board text added: "C15"
- board text added: "C16"
- board text added: "C17"
- board text added: "C18"
- board text added: "C19"
- board text added: "C2"
- board text added: "C20"
- board text added: "C21"
- board text added: "C22"
- board text added: "C23"
- board text added: "C24"
- board text added: "C25"
- board text added: "C26"
- board text added: "C27"
- board text added: "C28"
- board text added: "C29"
- board text added: "C3"
- board text added: "C30"
- board text added: "C31"
- board text added: "C32"
- board text added: "C33"
- board text added: "C34"
- board text added: "C35"
- board text added: "C36"
- board text added: "C4"
- board text added: "C5"
- board text added: "C6"
- board text added: "C7"
- board text added: "C8"
- board text added: "C9"
- board text added: "CVBS"
- board text added: "D1"
- board text added: "D2"
- board text added: "D3"
- board text added: "D4"
- board text added: "D5"
- board text added: "EAR"
- board text added: "J10"
- board text added: "J11"
- board text added: "J12"
- board text added: "J16"
- board text added: "JOY"
- board text added: "JTAG"
- board text added: "L1"
- board text added: "L2"
- board text added: "L3"
- board text added: "PS/2"
- board text added: "PWCON"
- board text added: "PWSW"
- board text added: "PWUSB"
- board text added: "R1"
- board text added: "R10"
- board text added: "R11"
- board text added: "R12"
- board text added: "R13"
- board text added: "R14"
- board text added: "R15"
- board text added: "R16"
- board text added: "R17"
- board text added: "R18"
- board text added: "R19"
- board text added: "R2"
- board text added: "R20"
- board text added: "R21"
- board text added: "R22"
- board text added: "R23"
- board text added: "R24"
- board text added: "R25"
- board text added: "R26"
- board text added: "R27"
- board text added: "R28"
- board text added: "R29"
- board text added: "R3"
- board text added: "R30"
- board text added: "R31"
- board text added: "R32"
- board text added: "R4"
- board text added: "R5"
- board text added: "R6"
- board text added: "R7"
- board text added: "R8"
- board text added: "R9"
- board text added: "RGB"
- board text added: "RST"
- board text added: "T1"
- board text added: "U1"
- board text added: "U2"
- board text added: "U3"
- board text added: "U4"
- board text added: "U5"
- board text added: "U6"
- board text added: "U7"
- board text added: "Y1"
- board text added: "Y2"
- board text added: "v4.1"
